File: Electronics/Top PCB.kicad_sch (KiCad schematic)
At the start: 3 parts

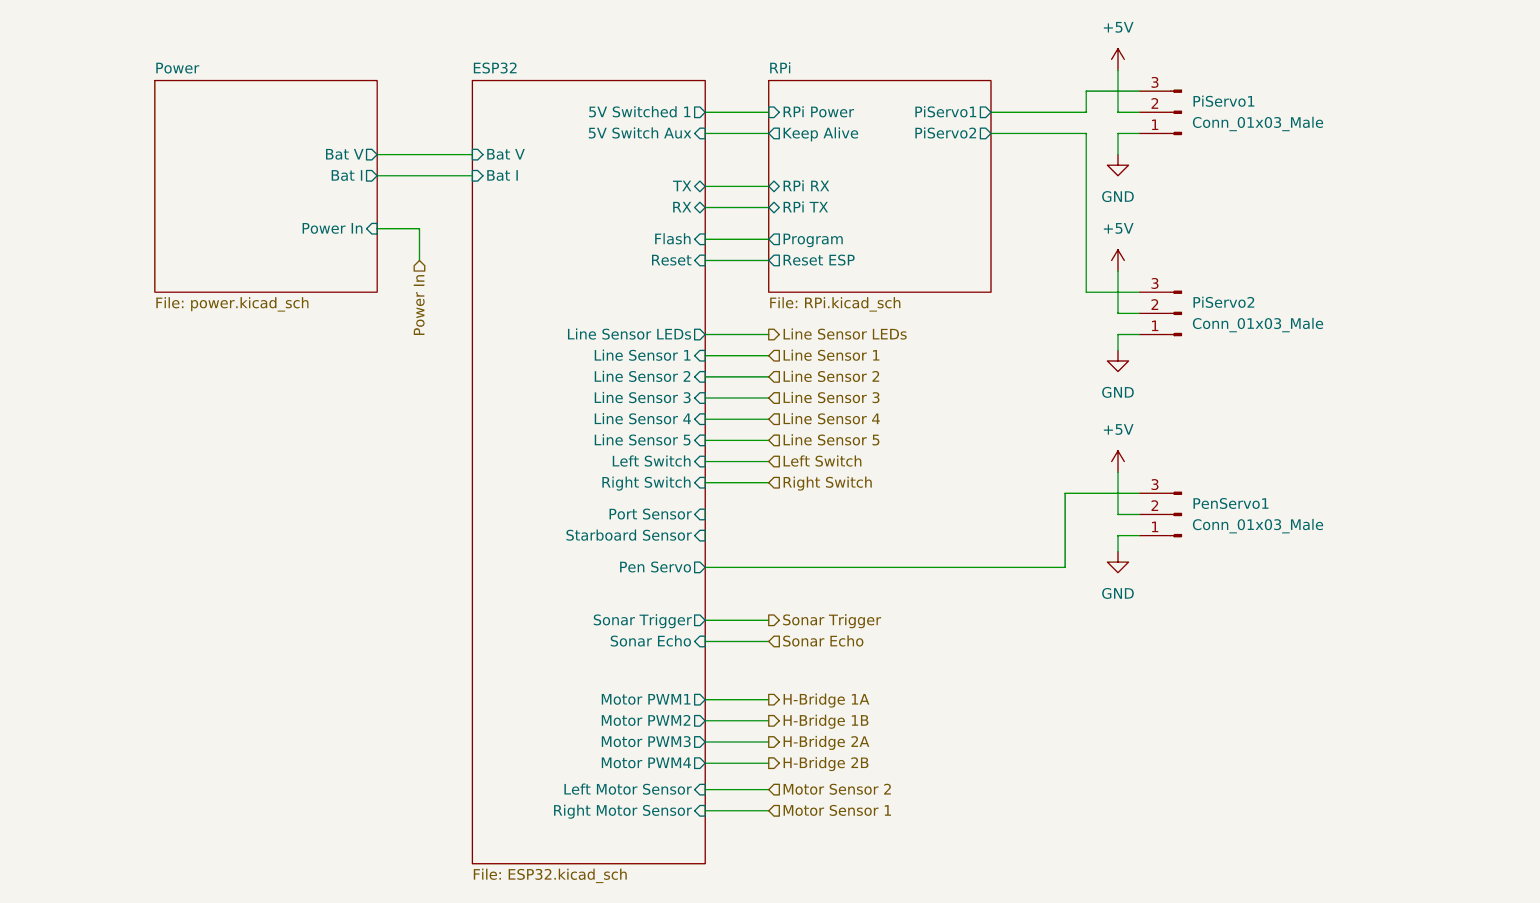
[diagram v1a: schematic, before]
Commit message: yep
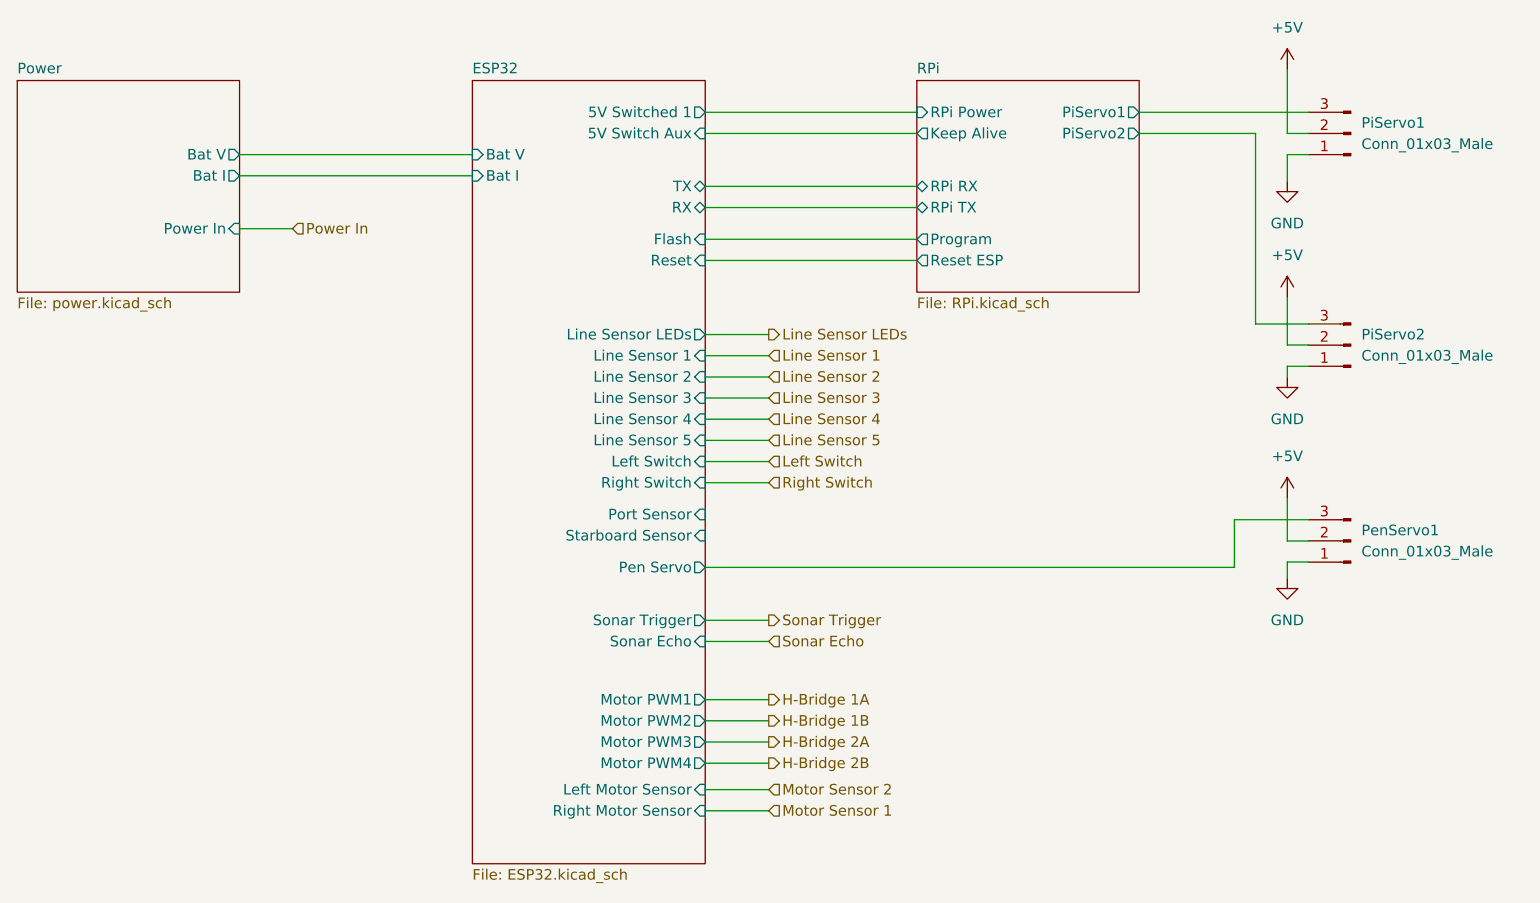
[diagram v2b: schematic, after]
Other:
- moved on the sheet: PenServo1, PiServo1, PiServo2

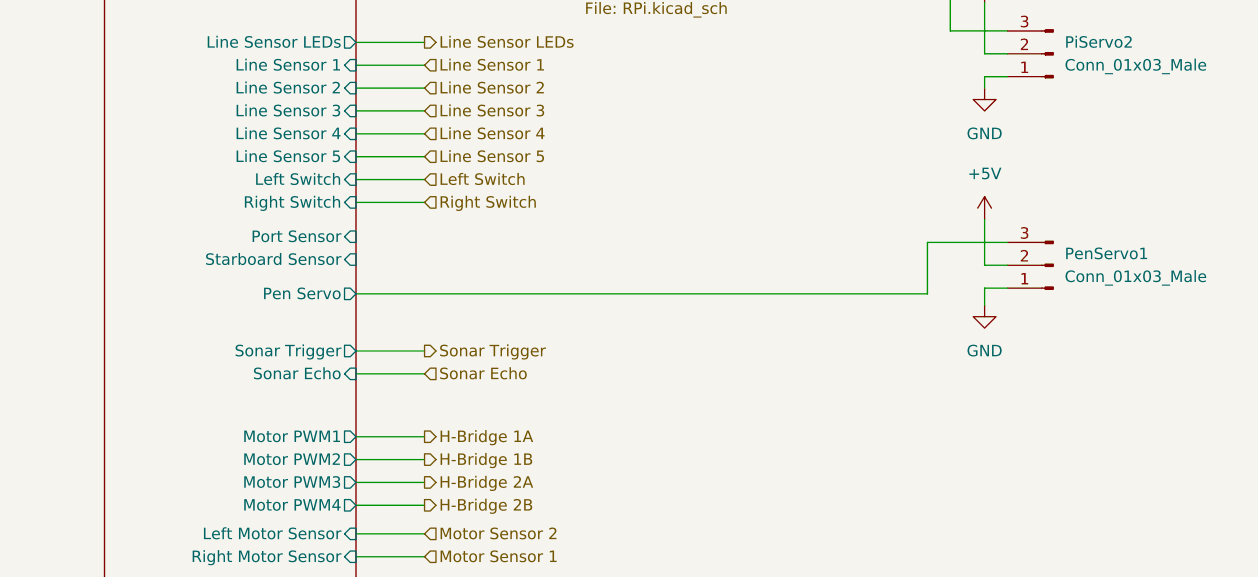
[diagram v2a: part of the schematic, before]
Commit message: some changes were made
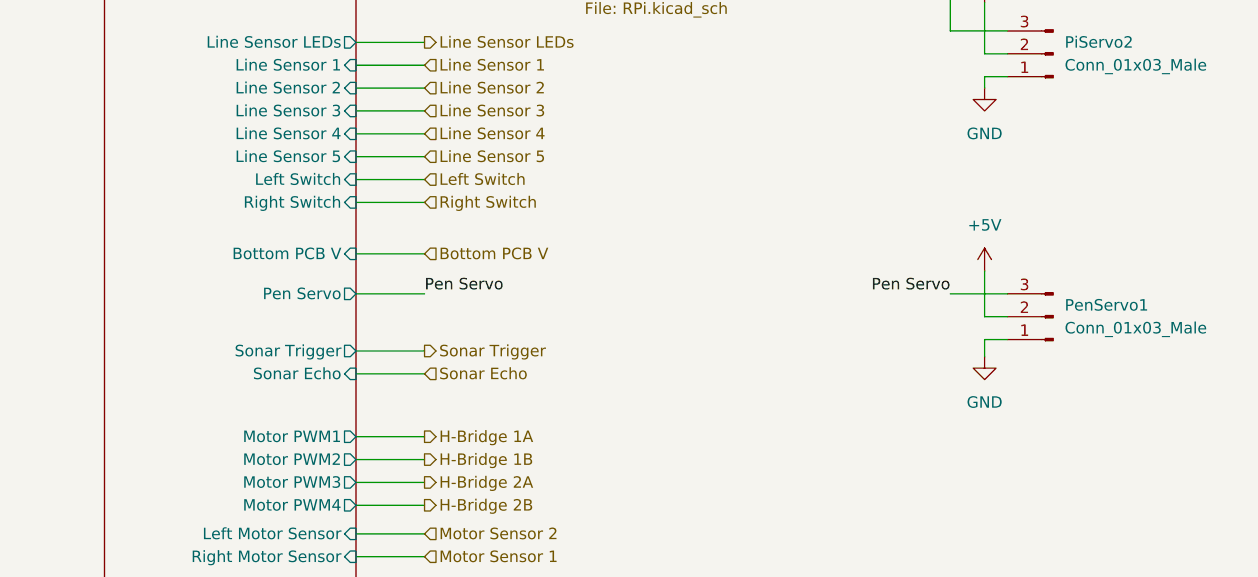
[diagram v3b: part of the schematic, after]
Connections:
- net ESP32/Pen Servo renamed Pen Servo
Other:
- sheet ESP32 ports: added Bottom PCB V; removed Port Sensor, Starboard Sensor
- company: (none) -> Squashed Fly
- title: (none) -> Swarmbot
- moved on the sheet: PenServo1
